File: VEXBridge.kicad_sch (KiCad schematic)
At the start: 56 parts, among them J1 4P4C, J10 QWIIC Connector, J11 QWIIC Connector, J12 QWIIC Connector, J13 QWIIC Connector, J14 QWIIC Connector, J15 4P4C, J2 Conn_01x04, J3 Conn_01x04, J4 QWIIC Connector, J5 QWIIC Connector, J6 Conn_01x04, J7 Conn_01x04, J8 USB_C_Receptacle_USB2.0_14P, J9 QWIIC Connector, U1 PCA9548ADB, U2 ESP32-S3-MINI-1U, U4 AMS1117-3.3, U5 LM2595S-5, U6 ISM330DHCX

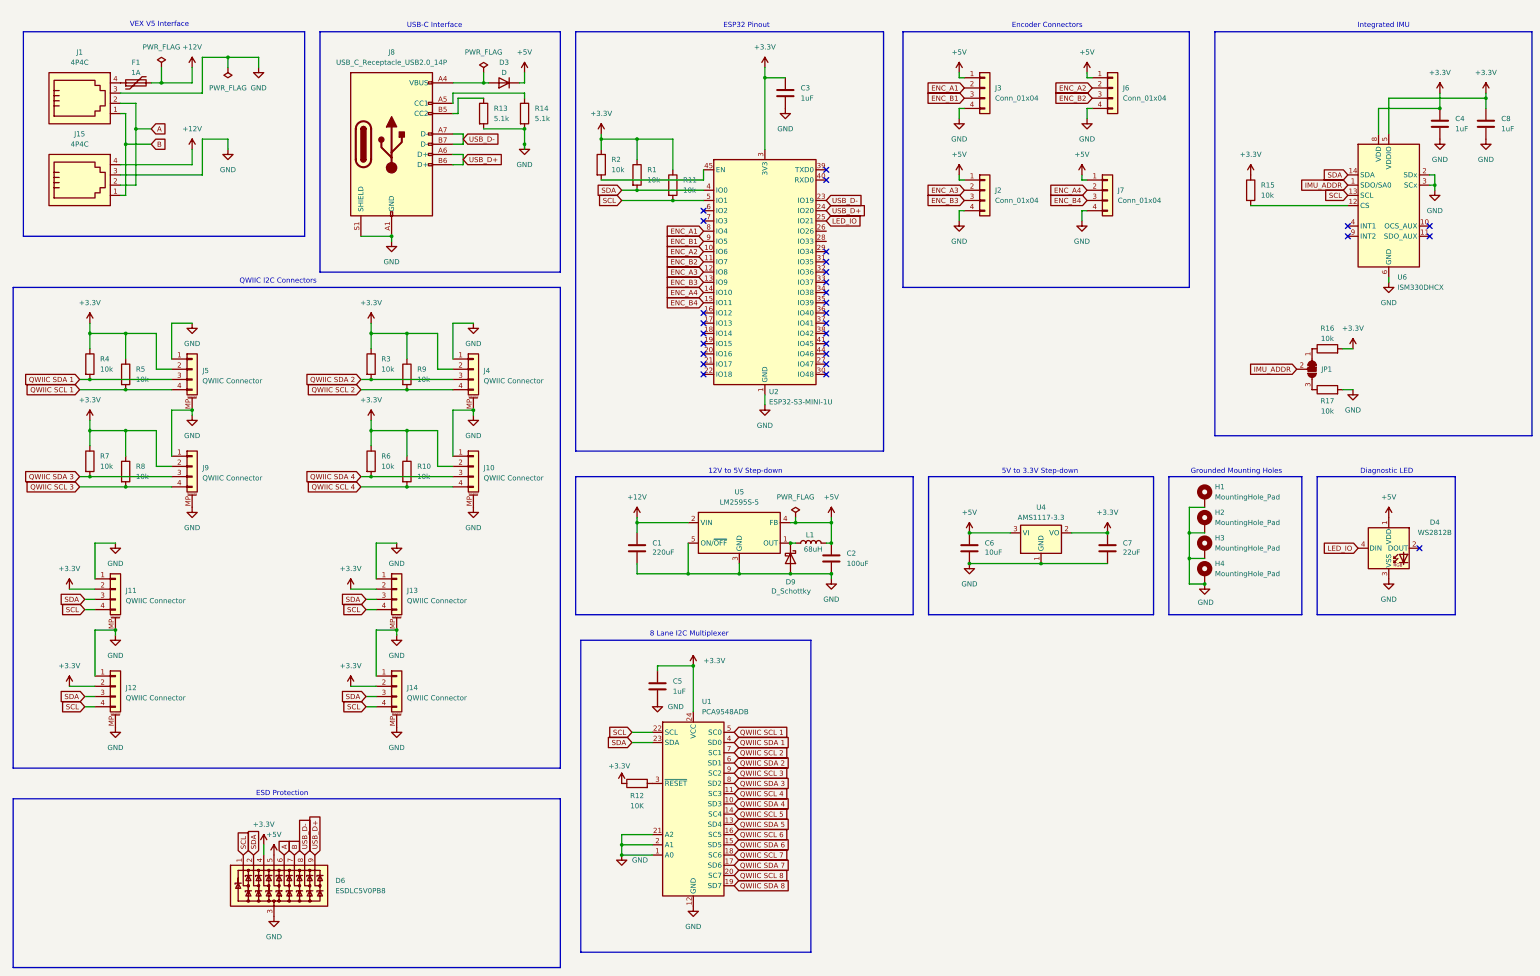
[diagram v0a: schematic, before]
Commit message: Completed schematic
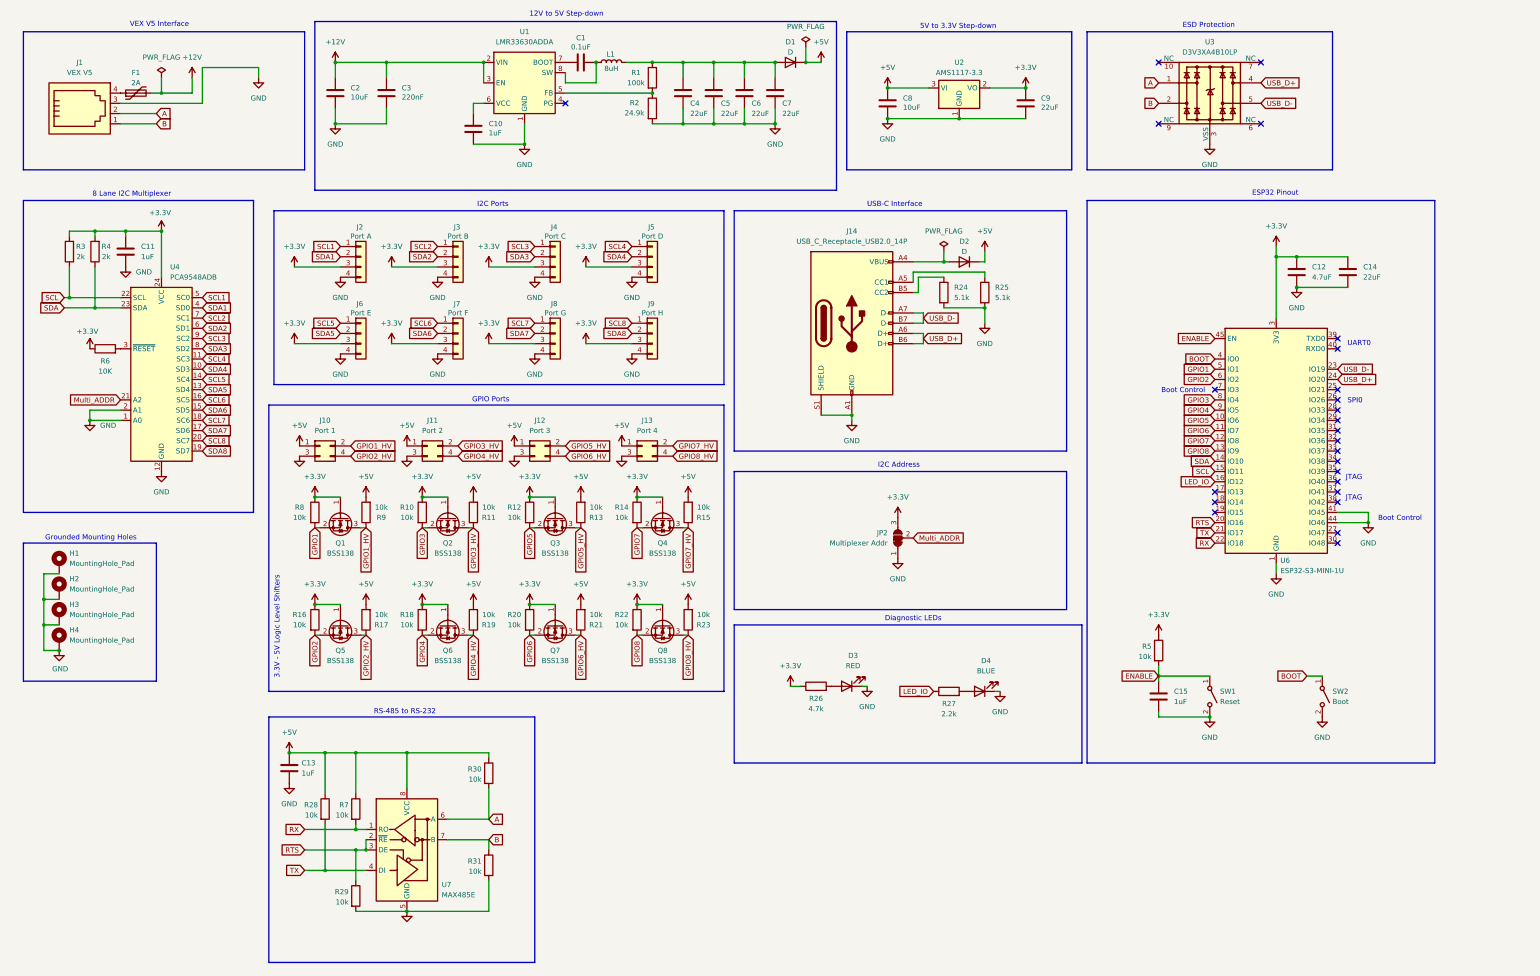
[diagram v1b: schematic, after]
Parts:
- removed C8: 1uF, Capacitor_SMD:C_0201_0603Metric, symbol Device:C
- removed D4: WS2812B, LED_SMD:LED_WS2812B_PLCC4_5.0x5.0mm_P3.2mm, symbol LED:WS2812B
- removed D6: ESDLC5V0PB8, Package_DFN_QFN:UDFN-9_1.0x3.8mm_P0.5mm, symbol Power_Protection:ESDLC5V0PB8
- removed D9: D_Schottky, Diode_SMD:D_SMA, symbol Device:D_Schottky
- removed J10, J11, J12, J13, J14, J4, J5, J9: QWIIC Connector, Connector_JST:JST_SH_SM04B-SRSS-TB_1x04-1MP_P1.00mm_Horizontal, symbol Connector_Generic_MountingPin:Conn_01x04_MountingPin
- removed J15: 4P4C, Connector_RJ:RJ9_Evercom_5301-440xxx_Horizontal, symbol Connector:4P4C
- removed JP1: SolderJumper_3_Bridged12, symbol Jumper:SolderJumper_3_Bridged12
- removed R6: 10k, Resistor_SMD:R_0805_2012Metric, symbol Device:R
- removed U5: LM2595S-5, Package_TO_SOT_SMD:TO-263-5_TabPin3, symbol Regulator_Switching:LM2595S-5
- removed U6: ISM330DHCX, Package_LGA:LGA-14_3x2.5mm_P0.5mm_LayoutBorder3x4y, symbol Sensor_Motion:ISM330DHCX
- added C10: 1uF, Capacitor_SMD:C_1210_3225Metric, symbol Device:C
- added C13, C15: 1uF, Capacitor_SMD:C_0201_0603Metric, symbol Device:C
- added C14: 22uF, Capacitor_SMD:C_0201_0603Metric, symbol Device:C
- added C3: 220nF, Capacitor_SMD:C_1210_3225Metric, symbol Device:C
- added C5, C6, C7: 22uF, Capacitor_SMD:C_1206_3216Metric, symbol Device:C
- added D1: D, Diode_SMD:D_0201_0603Metric, symbol Device:D
- added D3: RED, symbol Device:LED
- added D4: BLUE, symbol Device:LED
- added J10: Port 1, Connector_Molex:Molex_Mini-Fit_Jr_5569-04A2_2x02_P4.20mm_Horizontal, symbol Connector_Generic:Conn_02x02_Odd_Even
- added J11: Port 2, Connector_Molex:Molex_Mini-Fit_Jr_5569-04A2_2x02_P4.20mm_Horizontal, symbol Connector_Generic:Conn_02x02_Odd_Even
- added J12: Port 3, Connector_Molex:Molex_Mini-Fit_Jr_5569-04A2_2x02_P4.20mm_Horizontal, symbol Connector_Generic:Conn_02x02_Odd_Even
- added J13: Port 4, Connector_Molex:Molex_Mini-Fit_Jr_5569-04A2_2x02_P4.20mm_Horizontal, symbol Connector_Generic:Conn_02x02_Odd_Even
- added J4: Port C, Connector_JST:JST_SH_SM04B-SRSS-TB_1x04-1MP_P1.00mm_Horizontal, symbol Connector_Generic:Conn_01x04
- added J5: Port D, Connector_JST:JST_SH_SM04B-SRSS-TB_1x04-1MP_P1.00mm_Horizontal, symbol Connector_Generic:Conn_01x04
- added J8: Port G, Connector_JST:JST_SH_SM04B-SRSS-TB_1x04-1MP_P1.00mm_Horizontal, symbol Connector_Generic:Conn_01x04
- added J9: Port H, Connector_JST:JST_SH_SM04B-SRSS-TB_1x04-1MP_P1.00mm_Horizontal, symbol Connector_Generic:Conn_01x04
- added JP2: Multiplexer Addr, symbol Jumper:SolderJumper_3_Bridged12
- added Q1, Q2, Q3, Q4, Q5, Q6, Q7, Q8: BSS138, Package_TO_SOT_SMD:SOT-23, symbol Transistor_FET:BSS138
- added R12, R13, R14, R18, R19, R20, R21, R22, R23, R28, R29, R30, R31: 10k, Resistor_SMD:R_0805_2012Metric, symbol Device:R
- added R26: 4.7k, Resistor_SMD:R_0805_2012Metric, symbol Device:R
- added R27: 2.2k, Resistor_SMD:R_0805_2012Metric, symbol Device:R
- added SW1: Reset, symbol Switch:SW_SPST
- added SW2: Boot, symbol Switch:SW_SPST
- added U1: LMR33630ADDA, Package_SO:Texas_HSOP-8-1EP_3.9x4.9mm_P1.27mm_ThermalVias, symbol Regulator_Switching:LMR33630ADDA
- added U3: D3V3XA4B10LP, Package_DFN_QFN:Diodes_UDFN-10_1x2.5mm_P0.5mm, symbol Power_Protection:D3V3XA4B10LP
- added U7: MAX485E, Package_SO:SOIC-8_3.9x4.9mm_P1.27mm, symbol Interface_UART:MAX485E
- C1: value 220uF -> 0.1uF
- C12: renamed from C3; value 1uF -> 4.7uF
- C2: value 100uF -> 10uF; footprint Capacitor_SMD:C_1206_3216Metric -> Capacitor_SMD:C_1210_3225Metric
- C4: value 1uF -> 22uF; footprint Capacitor_SMD:C_0201_0603Metric -> Capacitor_SMD:C_1206_3216Metric
- F1: value 1A -> 2A
- J1: value 4P4C -> VEX V5
- J2: value Conn_01x04 -> Port A; footprint Connector_Molex:Molex_PicoBlade_53047-0410_1x04_P1.25mm_Vertical -> Connector_JST:JST_SH_SM04B-SRSS-TB_1x04-1MP_P1.00mm_Horizontal
- J3: value Conn_01x04 -> Port B; footprint Connector_Molex:Molex_PicoBlade_53047-0410_1x04_P1.25mm_Vertical -> Connector_JST:JST_SH_SM04B-SRSS-TB_1x04-1MP_P1.00mm_Horizontal
- J6: value Conn_01x04 -> Port E; footprint Connector_Molex:Molex_PicoBlade_53047-0410_1x04_P1.25mm_Vertical -> Connector_JST:JST_SH_SM04B-SRSS-TB_1x04-1MP_P1.00mm_Horizontal
- J7: value Conn_01x04 -> Port F; footprint Connector_Molex:Molex_PicoBlade_53047-0410_1x04_P1.25mm_Vertical -> Connector_JST:JST_SH_SM04B-SRSS-TB_1x04-1MP_P1.00mm_Horizontal
- L1: value 68uH -> 8uH; footprint Inductor_SMD:L_SXN_SMDRI127 -> Inductor_SMD:L_0603_1608Metric
- R1: value 10k -> 100k
- R2: value 10k -> 24.9k
- R3, R4: value 10k -> 2k
- R6: renamed from R12; footprint (none) -> Resistor_SMD:R_0805_2012Metric
- renumbered C5 to C11, C6 to C8, C7 to C9, D3 to D2, J8 to J14, R13 to R24, R14 to R25, U4 to U2, U1 to U4, U2 to U6
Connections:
- net QWIIC SDA 6 is gone; now on net SDA6: U4.15 (SD5)
- net +12V: now also C2.1, C3.1, U1.2 (VIN), U1.3 (EN); no longer C1.1
- net +3.3V: now also J2.3 (Pin_3), J3.3 (Pin_3), J6.3 (Pin_3), J7.3 (Pin_3), R16.1, R3.2, R4.2, C14.1, J4.3 (Pin_3), J5.3 (Pin_3), J8.3 (Pin_3), J9.3 (Pin_3), JP2.3 (B), Q1.1 (G), Q2.1 (G), Q3.1 (G), Q4.1 (G), Q5.1 (G), Q6.1 (G), Q7.1 (G), Q8.1 (G), R12.1, R14.1, R18.1, R20.1, R22.1, R26.1; no longer C4.1, R1.1, R11.1, R15.1, R16.2, R2.1, R3.1, R4.1, R7.1, R9.1
- net +5V: now also R11.2, R15.2, R17.2, R7.1, R9.2, C13.1, D1.1 (K), J10.1 (Pin_1), J11.1 (Pin_1), J12.1 (Pin_1), J13.1 (Pin_1), R13.2, R19.2, R21.2, R23.2, R28.1, R30.1, U7.8 (VCC); no longer C2.1, J2.1 (Pin_1), J3.1 (Pin_1), J6.1 (Pin_1), J7.1 (Pin_1), L1.2
- net A: now also R30.2, U3.1, U7.6 (A)
- net B: now also R31.1, U3.2, U7.7 (B)
- net GND: now also R2.2, U6.41 (IO45), U6.44 (IO46), C10.2, C13.2, C14.2, C15.2, C3.2, C5.2, C6.2, C7.2, D3.1 (K), D4.1 (K), J10.3 (Pin_3), J11.3 (Pin_3), J12.3 (Pin_3), J13.3 (Pin_3), J4.4 (Pin_4), J5.4 (Pin_4), J8.4 (Pin_4), J9.4 (Pin_4), JP2.1 (A), R29.2, R31.2, SW1.2 (B), SW2.2 (B), U1.1 (GND), U1.9 (GND), U3.3 (VSS), U3.8 (VSS), U7.5 (GND); no longer C1.2, R17.2, U4.21 (A2)
- net LED_IO: now also U6.16 (IO12), R27.1; no longer U6.25 (IO21)
- net SCL: now also R3.1, U6.15 (IO11); no longer R11.2, U6.5 (IO1)
- net SDA: now also R4.1, U6.14 (IO10); no longer R1.2, U6.4 (IO0)
- net USB_D+: now also U3.4
- net USB_D-: now also U3.5
- net at L1.1: now also C1.2, U1.8 (SW)
- net GPIO2_HV: now reaches R17.1
- net GPIO2_HV: now also J10.4 (Pin_4), Q5.3 (D)
- net RTS: now reaches U6.20 (IO16)
- net RTS: now also R29.1, U7.2 (~{RE}), U7.3 (DE)
- net TX: now reaches U6.21 (IO17)
- net TX: now also R28.2, U7.4 (DI)
- net RX: now reaches U6.22 (IO18)
- net RX: now also R7.2, U7.1 (RO)
- net ENABLE: now reaches U6.45 (EN)
- net ENABLE: now also R5.2, C15.1, SW1.1 (A); no longer R2.2
- net GPIO2: now reaches U6.6 (IO2)
- net GPIO2: now also R16.2, Q5.2 (S)
- net ENC_A1 renamed GPIO3
- net GPIO3: now also R10.2, Q2.2 (S); no longer J3.2 (Pin_2)
- net ENC_A2 renamed GPIO5
- net GPIO5: now also Q3.2 (S), R12.2; no longer J6.2 (Pin_2)
- net ENC_A3 renamed GPIO7
- net GPIO7: now also Q4.2 (S), R14.2; no longer J2.2 (Pin_2)
- net ENC_A4 renamed SDA6
- net SDA6: no longer U6.14 (IO10)
- net ENC_B1 renamed GPIO4
- net GPIO4: now also Q6.2 (S), R18.2; no longer J3.3 (Pin_3)
- net ENC_B2 renamed GPIO6
- net GPIO6: now also Q7.2 (S), R20.2; no longer J6.3 (Pin_3)
- net ENC_B3 renamed GPIO8
- net GPIO8: now also Q8.2 (S), R22.2; no longer J2.3 (Pin_3)
- removed net ENC_B4: J7.3 (Pin_3), U6.15 (IO11)
- net QWIIC SCL 1 renamed SCL1
- net SCL1: now also J2.1 (Pin_1); no longer R5.2
- net QWIIC SCL 2 renamed SCL2
- net SCL2: now also J3.1 (Pin_1); no longer R9.2
- net QWIIC SCL 3 renamed GPIO1
- net GPIO1: now also U6.5 (IO1), Q1.2 (S); no longer U4.9 (SC2)
- net QWIIC SCL 4 renamed SCL4
- net SCL4: now also J5.1 (Pin_1); no longer R10.2
- net QWIIC SCL 5 renamed SCL5
- net SCL5: now also J6.1 (Pin_1)
- net QWIIC SCL 6 renamed SCL6
- net SCL6: now also J7.1 (Pin_1)
- net QWIIC SCL 7 renamed SCL7
- net SCL7: now also J8.1 (Pin_1)
- net QWIIC SCL 8 renamed SCL8
- net SCL8: now also J9.1 (Pin_1)
- net QWIIC SDA 1 renamed SDA1
- net SDA1: now also J2.2 (Pin_2); no longer R4.2
- net QWIIC SDA 2 renamed SDA2
- net SDA2: now also J3.2 (Pin_2); no longer R3.2
- net QWIIC SDA 3 renamed SDA3
- net SDA3: now also J4.2 (Pin_2); no longer R7.2
- net QWIIC SDA 4 renamed SDA4
- net SDA4: now also J5.2 (Pin_2)
- net QWIIC SDA 5 renamed SDA5
- net SDA5: now also J6.2 (Pin_2)
- net QWIIC SDA 7 renamed SDA7
- net SDA7: now also J8.2 (Pin_2)
- net QWIIC SDA 8 renamed SDA8
- net SDA8: now also J9.2 (Pin_2)
- new net: C4.1, C5.1, C6.1, C7.1, D1.2 (A), L1.2, R1.1
- new net: D4.2 (A), R27.2
- new net: D3.2 (A), R26.2
- new net: R1.2, R2.1, U1.5 (FB)
- new net: C10.1, U1.6 (VCC)
- new net: C1.1, U1.7 (BOOT)
- new net BOOT: SW2.1 (A), U6.4 (IO0)
- new net GPIO1_HV: J10.2 (Pin_2), Q1.3 (D), R9.1
- new net GPIO3_HV: J11.2 (Pin_2), Q2.3 (D), R11.1
- new net GPIO4_HV: J11.4 (Pin_4), Q6.3 (D), R19.1
- new net GPIO5_HV: J12.2 (Pin_2), Q3.3 (D), R13.1
- new net GPIO6_HV: J12.4 (Pin_4), Q7.3 (D), R21.1
- new net GPIO7_HV: J13.2 (Pin_2), Q4.3 (D), R15.1
- new net GPIO8_HV: J13.4 (Pin_4), Q8.3 (D), R23.1
- new net Multi_ADDR: JP2.2 (C), U4.21 (A2)
- new net SCL3: J4.1 (Pin_1), U4.9 (SC2)
- no-connect marks 29 -> 25
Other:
- note added: "3.3V - 5V Logic Level Shifters"
- note added: "Boot Control"
- note added: "Diagnostic LEDs"
- note added: "GPIO Ports"
- note added: "I2C Address"
- note added: "I2C Ports"
- note added: "JTAG"
- note added: "RS-485 to RS-232"
- note added: "SPI0"
- note added: "UART0"
- note removed: "Diagnostic LED"
- note removed: "Encoder Connectors"
- note removed: "Integrated IMU"
- note removed: "QWIIC I2C Connectors"
- moved on the sheet: C11, C12, C8, C9, D2, F1, H1, H2, H3, H4, J1, J14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
